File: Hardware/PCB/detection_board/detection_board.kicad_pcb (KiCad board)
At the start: 2 copper layers, 60 x 50 mm, 32 parts, among them J1 DE9_Pins, U1 MICROFC-60035-SMT-TR1, U2 LT1807, U3 ADCMP601, U4 OPA365, U5 TS12A4514DBVR

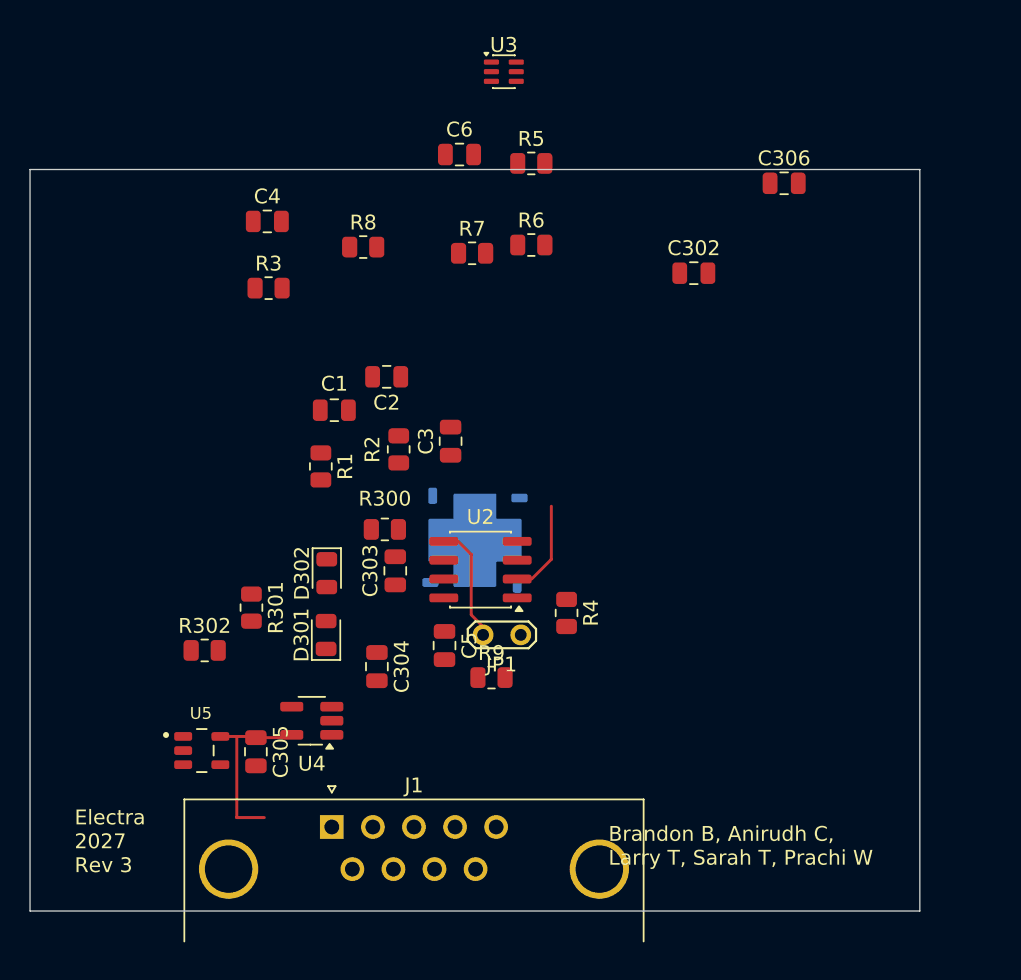
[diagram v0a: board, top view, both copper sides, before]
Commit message: Board layout
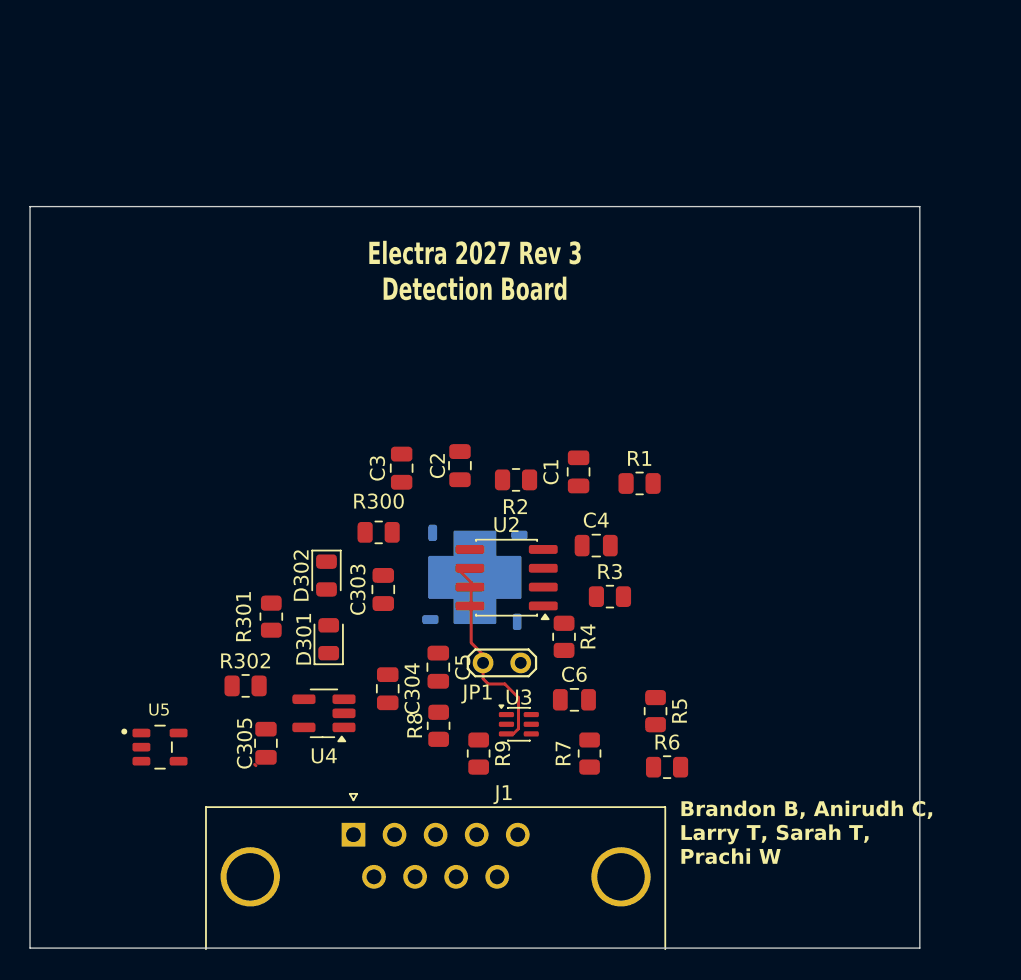
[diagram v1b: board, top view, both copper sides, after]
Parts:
- removed C302: 10n, Capacitor_SMD:C_0805_2012Metric
- removed C306: 100n, Capacitor_SMD:C_0805_2012Metric
- moved U3 44.0 mm to (171.0, 89.9)
- moved R5 37.9 mm to (180.2, 89.0), turned to -90 degrees
- moved C6 37.6 mm to (174.7, 88.3)
- moved R6 36.4 mm to (181.0, 92.8)
- moved R7 34.7 mm to (175.7, 91.9), turned to -90 degrees
- moved R8 32.7 mm to (165.6, 90.0), turned to -90 degrees
- moved C4 31.1 mm to (176.2, 77.9)
- moved R3 31.0 mm to (177.1, 81.3)
- moved R1 21.5 mm to (179.1, 73.7), turned to 0 degrees
- moved C1 17.0 mm to (175.0, 72.9), turned to -90 degrees
- moved R2 8.18 mm to (170.8, 73.4), turned to 180 degrees
- moved C2 7.76 mm to (167.0, 72.5), turned to -90 degrees
- moved R9 5.20 mm to (168.2, 91.9), turned to -90 degrees
- moved C3 3.77 mm to (163.1, 72.6)
- moved R302 3.65 mm to (152.5, 87.3)
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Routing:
- net +3V3: track 12.3 -> 0.00 mm
- net /peak_detect/pm_in: track 6.59 -> 13.6 mm
- net Net-(U2A--): track 5.46 -> 0.00 mm
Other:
- board text added: "Electra 2027 Rev 3 Detection Board"
- board text removed: "Electra 2027 Rev 3"
